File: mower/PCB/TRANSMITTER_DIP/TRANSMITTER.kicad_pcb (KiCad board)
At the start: 2 copper layers, 63 x 32.8 mm, 16 parts, among them J1 BOT POWER, J2 POWER IN, J3 SHUNT, J4 COIL OUT, J5 COIL POWER IN, Q1 IRF3205, U1 LM358, U4 LM555xN

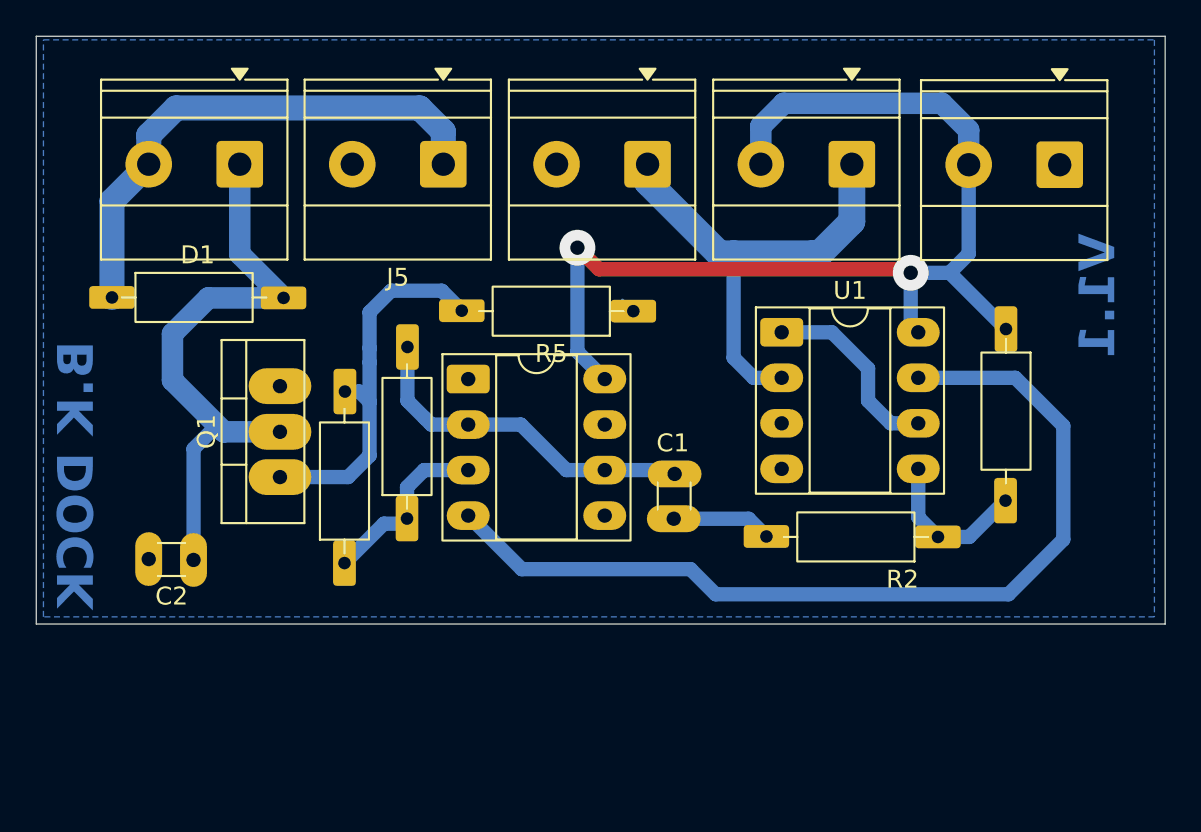
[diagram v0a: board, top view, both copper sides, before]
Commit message: Consolidate complete mower design (all branches) + zana repo structure
Mower fragments from every botkorp branch (mowbot3/4, TRANSMITTER_SMD,
IMRANS_LIBRARY) unioned into mower/. Adds legacy/opengro, README, .gitignore.
Sits on top of the preserved 13-commit mower history.

Co-Authored-By: Claude Opus 4.8 <noreply@anthropic.com>
Claude-Session: https://claude.ai/code/session_017QXBEryTihUadNUZqQzfmo
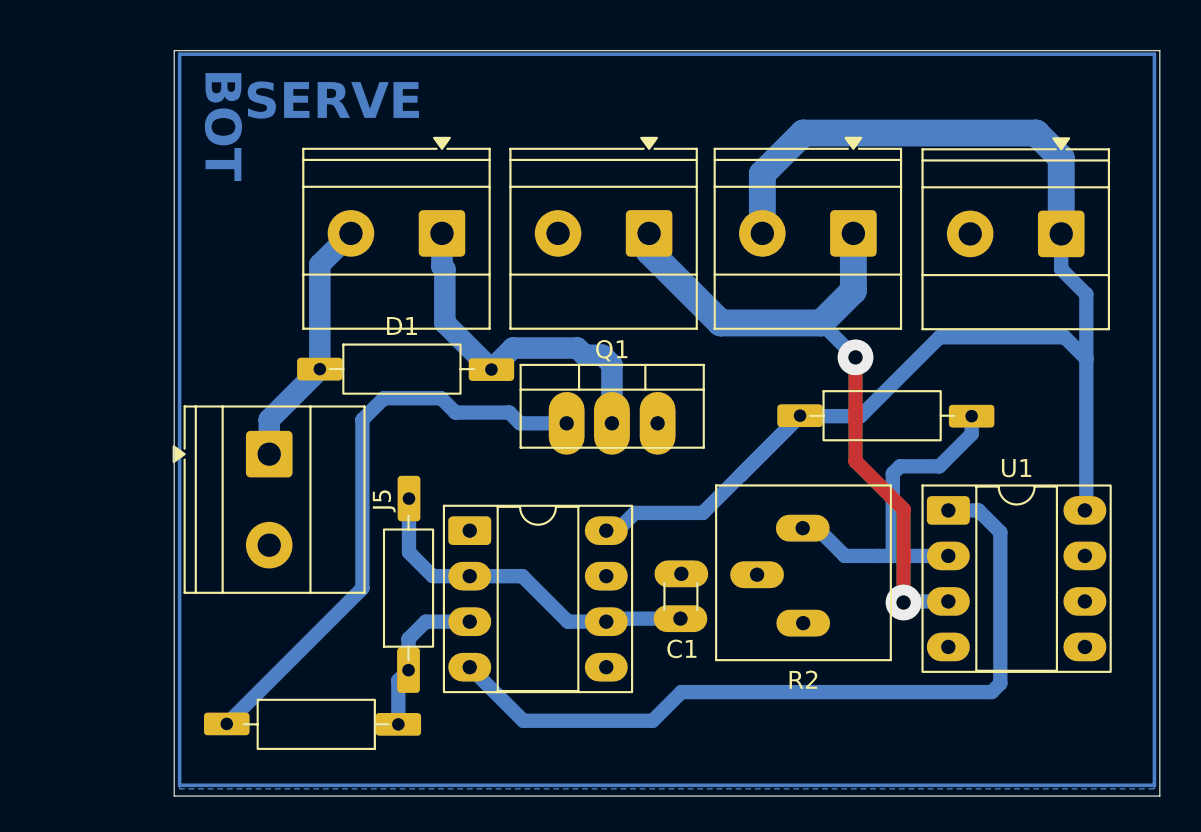
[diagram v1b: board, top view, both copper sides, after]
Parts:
- removed C2: 100nF, IMRANS_LIBRARY:C_Disc_D3.0mm_W1.6mm_P2.50mm
- removed R5: 1K, IMRANS_LIBRARY:R_Axial_DIN0207_L6.3mm_D2.5mm_P10.16mm_Horizontal_2
- D1: value 1N4007 -> 1N5819
- R1: value 10K -> 10k
- R2: value 10K -> 10k; footprint IMRANS_LIBRARY:R_Axial_DIN0207_L6.3mm_D2.5mm_P10.16mm_Horizontal_2 -> IMRANS_LIBRARY:Potentiometer_Bourns_3386P_Vertical
- moved J5 18.9 mm to (107.8, 57.5), turned to -90 degrees
- moved Q1 16.3 mm to (124.4, 55.8), turned to 0 degrees
- moved U1 13.6 mm to (145.7, 60.7)
- moved R1 13.1 mm to (136.9, 55.4), turned to 0 degrees
- moved D1 12.3 mm to (110.1, 52.8)
- moved J4 11.9 mm to (117.4, 45.2)
- moved R4 9.19 mm to (115.5, 72.6), turned to 180 degrees
- moved R3 8.46 mm to (115.6, 70.1)
- moved U4 8.46 mm to (119.0, 61.8)
- moved C1 8.13 mm to (130.8, 66.7), turned to 90 degrees
- moved R2 8.04 mm to (137.6, 61.6)
- moved J1 3.86 mm to (129.0, 45.2)
- moved J2 3.86 mm to (152.0, 45.2)
- moved J3 3.86 mm to (140.4, 45.2)
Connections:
- J2 pad 1: GND -> VCC
- J2 pad 2: VCC -> GND
- R1 pad 2: Net-(U1B-+) -> Net-(U1A--)
- R2 pad 1: Net-(U1B-+) -> Net-(U1A--)
- U1 pad 1: Net-(U1B--) -> Net-(U4-R)
- U1 pad 2: Net-(J1-Pin_1) -> Net-(U1A--)
- U1 pad 3: GND -> Net-(J1-Pin_1)
- U1 pad 5: Net-(U1B-+) -> (no net)
- U1 pad 6: Net-(U1B--) -> (no net)
- U1 pad 7: Net-(U4-R) -> (no net)
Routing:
- net Net-(U1A--): track 0.00 -> 18.9 mm
- net VCC: track 60.5 -> 79.1 mm, vias 2 -> 0
- net VCOIL: track 29.3 -> 14.2 mm
- net Net-(D1-A): track 33.6 -> 20.3 mm
- net Net-(Q1-G): track 21.2 -> 34.0 mm
- net Net-(J1-Pin_1): track 27.0 -> 38.0 mm, vias 0 -> 2
- net Net-(U1B--): track 10.8 -> 0.00 mm
- net Net-(U1B-+): track 8.86 -> 0.00 mm
- net Net-(U4-R): track 51.8 -> 43.6 mm
- net GND: track 7.19 -> 0.00 mm
- net Net-(U4-Q): track 10.1 -> 8.82 mm
- net Net-(U4-THR): track 19.8 -> 20.6 mm
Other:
- board size 63 x 32.8 mm -> 55 x 41.6 mm
- board text added: "BOT"
- board text added: "SERVE"
- board text removed: "B.K DOCK"
- board text removed: "V1.1"
